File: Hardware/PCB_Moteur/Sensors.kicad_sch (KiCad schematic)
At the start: 19 parts, among them J18 Screw_Terminal_01x04, J19 Screw_Terminal_01x04, U7 INA125UA/2K5, U8 INA125UA/2K5, U9 MAX6612MXK

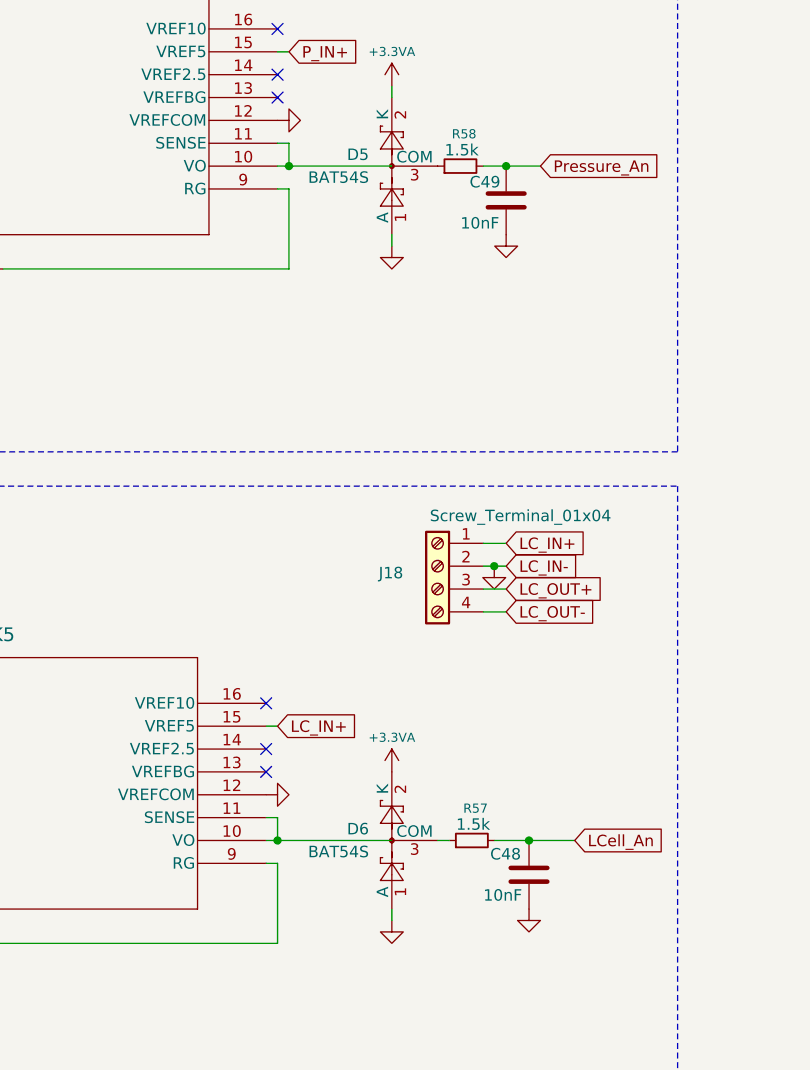
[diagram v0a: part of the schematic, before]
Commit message: wip: début routing
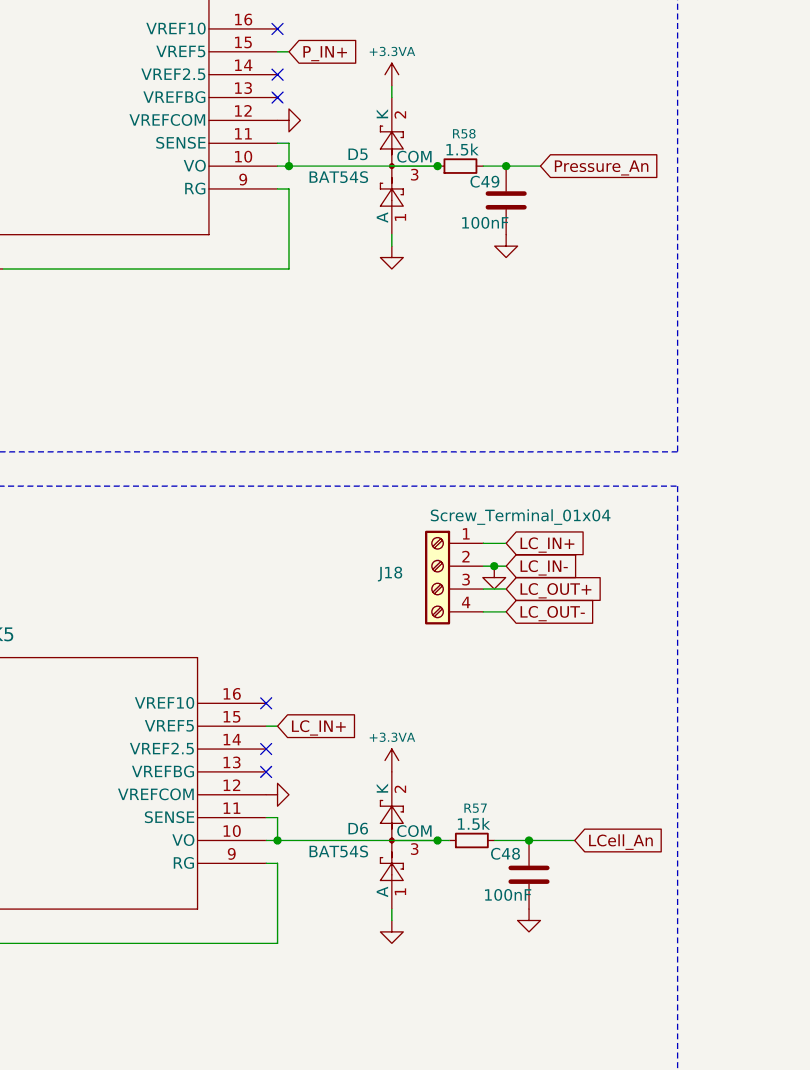
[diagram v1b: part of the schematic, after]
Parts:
- C48: value 10nF -> 100nF; footprint Capacitor_SMD:C_0603_1608Metric -> Capacitor_SMD:C_0805_2012Metric
- C49: value 10nF -> 100nF
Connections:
- net at D5.3 (COM), R58.1: now also U7.10 (VO), U7.11 (SENSE)
- net at D6.3 (COM), R57.1: now also U8.10 (VO), U8.11 (SENSE)
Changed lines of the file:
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@@
+	)
+	(junction
+		(at 142.24 140.97)
+		(diameter 0)
+		(color 0 0 0 0)
+	)
+	(junction
+		(at 220.98 49.53)
+		(diameter 0)
+		(color 0 0 0 0)
+	)
+	(junction
+		(at 34.29 128.27)
+		(diameter 0)
+		(color 0 0 0 0)
+	)
+	(junction
+		(at 132.08 66.04)
+		(diameter 0)
+		(color 0 0 0 0)
+	)
+	(junction
+		(at 139.7 66.04)
+		(diameter 0)
+		(color 0 0 0 0)
 	)
 	(junction
@@
 	)
 	(junction
-		(at 142.24 140.97)
+		(at 43.18 44.45)
 		(diameter 0)
 		(color 0 0 0 0)
 	)
 	(junction
-		(at 220.98 49.53)
-		(diameter 0)
-		(color 0 0 0 0)
-	)
-	(junction
-		(at 34.29 128.27)
-		(diameter 0)
-		(color 0 0 0 0)
-	)
-	(junction
-		(at 139.7 66.04)
-		(diameter 0)
-		(color 0 0 0 0)
-	)
-	(junction
-		(at 43.18 44.45)
+		(at 132.08 140.97)
 		(diameter 0)
 		(color 0 0 0 0)
@@
 	(wire
 		(pts
-			(xy 114.3 140.97) (xy 113.03 140.97)
-		)
-		(stroke
-			(width 0)
-			(type default)
-		)
-	)
-	(wire
-		(pts
 			(xy 257.81 39.37) (xy 269.24 39.37)
 		)
@@
 	(wire
 		(pts
-			(xy 114.3 140.97) (xy 127 140.97)
+			(xy 113.03 140.97) (xy 114.3 140.97)
 		)
 		(stroke
@@
 	(wire
 		(pts
+			(xy 114.3 140.97) (xy 132.08 140.97)
+		)
+		(stroke
+			(width 0)
+			(type default)
+		)
+	)
+	(wire
+		(pts
 			(xy 267.97 34.29) (xy 266.7 34.29)
 		)
@@
 	(wire
 		(pts
-			(xy 133.35 140.97) (xy 132.08 140.97)
-		)
-		(stroke
-			(width 0)
-			(type default)
-		)
-	)
-	(wire
-		(pts
 			(xy 43.18 50.8) (xy 43.18 44.45)
 		)
@@
 	(wire
 		(pts
+			(xy 132.08 140.97) (xy 133.35 140.97)
+		)
+		(stroke
+			(width 0)
+			(type default)
+		)
+	)
+	(wire
+		(pts
 			(xy 83.82 77.47) (xy 115.57 77.47)
 		)
@@
 	(wire
 		(pts
-			(xy 115.57 66.04) (xy 127 66.04)
+			(xy 115.57 66.04) (xy 132.08 66.04)
 		)
 		(stroke
@@
 			)
 		)
-		(property "Value" "10nF"
+		(property "Value" "100nF"
 			(at 134.62 72.39 0)
 			(effects
@@
 			)
 		)
-		(property "Value" "10nF"
+		(property "Value" "100nF"
 			(at 137.16 147.066 0)
 			(effects
@@
 			)
 		)
-		(property "Footprint" "Capacitor_SMD:C_0603_1608Metric"
+		(property "Footprint" "Capacitor_SMD:C_0805_2012Metric"
 			(at 143.2052 148.59 0)
 			(effects
